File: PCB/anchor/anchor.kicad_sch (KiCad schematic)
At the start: 37 parts, among them J1 TSM-102-01-X-SV, J2 Conn_ARM_JTAG_SWD_10, J3 SM02B-SRSS-TB LFSN, J4 TSM-102-01-X-SV, J5 TSM-102-01-X-SV, J6 TSM-102-01-X-SV, J7 TSM-102-01-X-SV, J8 TSM-102-01-X-SV, Q1 IRLML2402TRPBF, Q2 IRLML2402TRPBF, U1 Voltage Regulator, U2 DWM3001C UWB, U3 LYR998

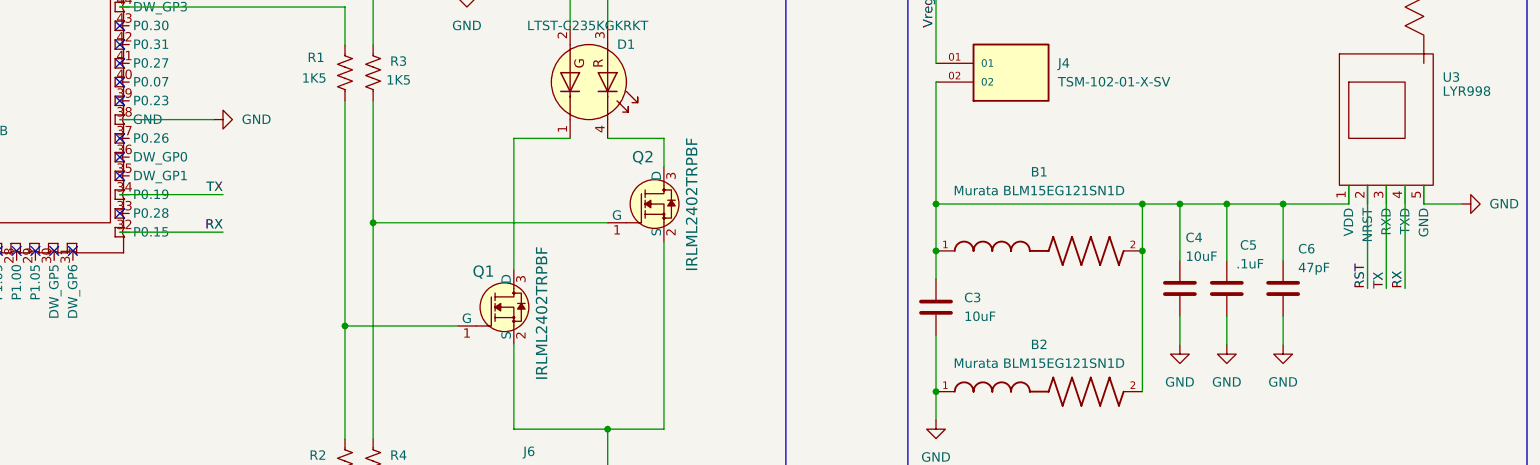
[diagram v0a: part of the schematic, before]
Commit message: update
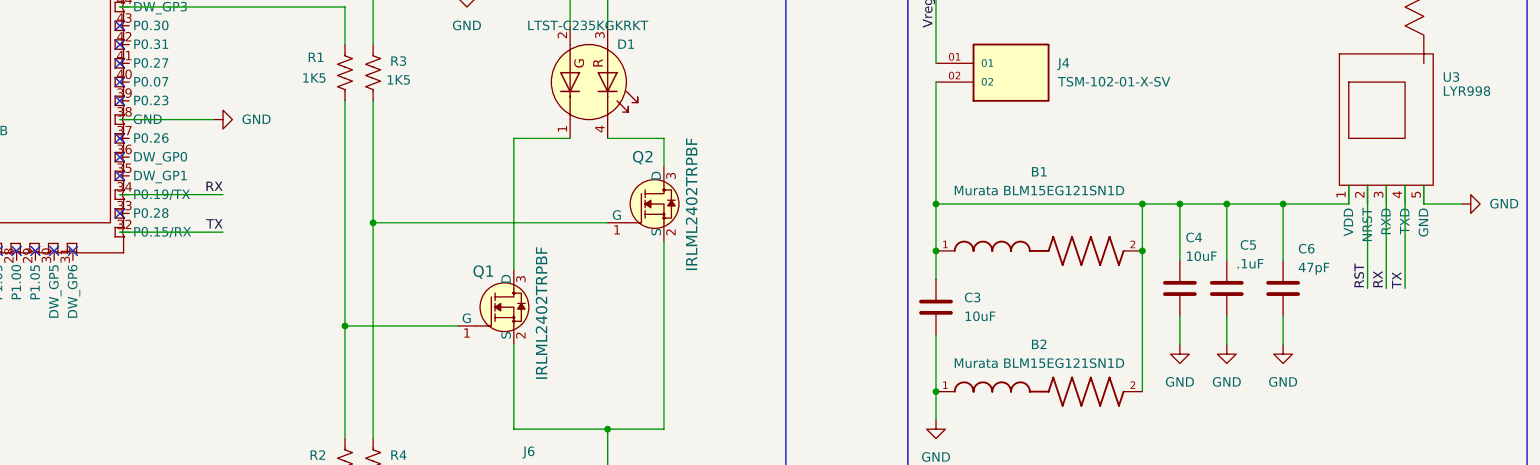
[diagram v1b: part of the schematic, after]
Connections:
- net RX: now also U2.34 (P0.19/TX), U3.3 (RXD); no longer U2.32 (P0.15), U3.4 (TXD)
- net TX: now also U2.32 (P0.15/RX), U3.4 (TXD); no longer U2.34 (P0.19), U3.3 (RXD)
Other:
- moved on the sheet: U2
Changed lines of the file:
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@@
 		)
 	)
-	(label "TX"
+	(label "RX"
 		(at 373.38 153.67 90)
 		(fields_autoplaced yes)
@@
 		)
 	)
-	(label "RX"
+	(label "TX"
 		(at 215.9 146.05 180)
 		(fields_autoplaced yes)
@@
 		)
 	)
-	(label "TX"
+	(label "RX"
 		(at 215.9 140.97 180)
 		(fields_autoplaced yes)
@@
 		)
 	)
-	(label "RX"
+	(label "TX"
 		(at 375.92 153.67 90)
 		(fields_autoplaced yes)

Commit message: PCB updates
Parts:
- C1: now not fitted
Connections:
- net Vreg: no longer J1.02, J2.1 (VTref), J4.01, J7.01, J8.01, R5.1, R6.1
- net Vbatt+3.3V: now reaches J5.02, U1.1 (IN), U1.3 (EN)
- net RX renamed RX (BIDIRECTIONAL)
- net SWD_CLK renamed SWD_CLK (IN)
- net SWD_CLK (IN): no longer J2.4 (SWCLK/TCK)
- net SWD_DIO renamed SWD_DIO (BIDIRECTIONAL)
- net TX renamed TX (BIDIRECTIONAL)
- new net SWD_CLK (OUT): J2.4 (SWCLK/TCK)
- new net Vreg +3.3V: J1.02, J2.1 (VTref), J4.01, J7.01, J8.01, R5.1, R6.1
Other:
- company: (none) -> Team 3
- moved on the sheet: B1, B2, C2, C3, C4, C5, C6, C7, C8, D1, D2, D3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
